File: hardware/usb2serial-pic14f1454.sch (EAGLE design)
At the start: 14 parts, among them IC1 PIC16F1454, IC2 LP2950-33, J1 USB-SHIELD-A-H, J2 J2

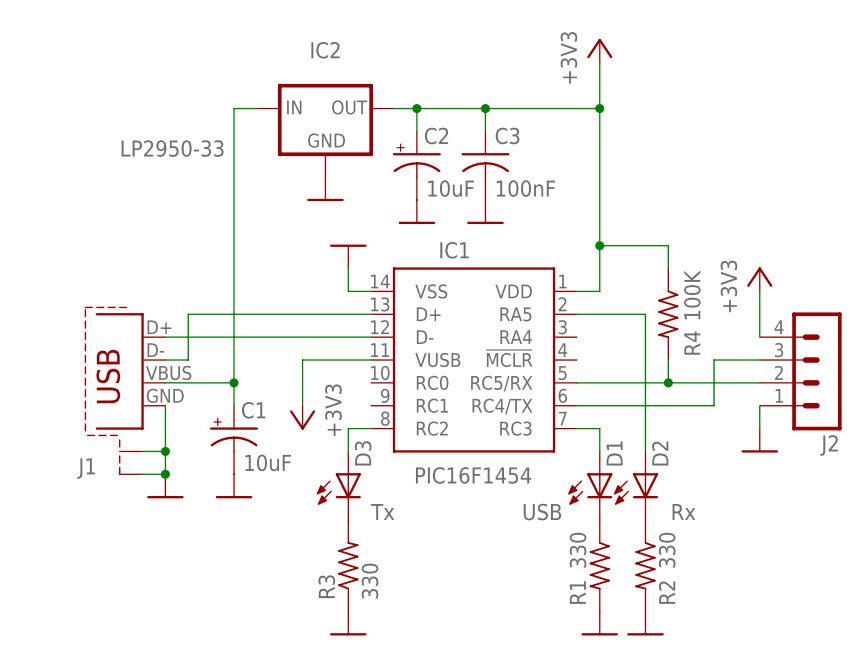
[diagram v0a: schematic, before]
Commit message: Cleanup
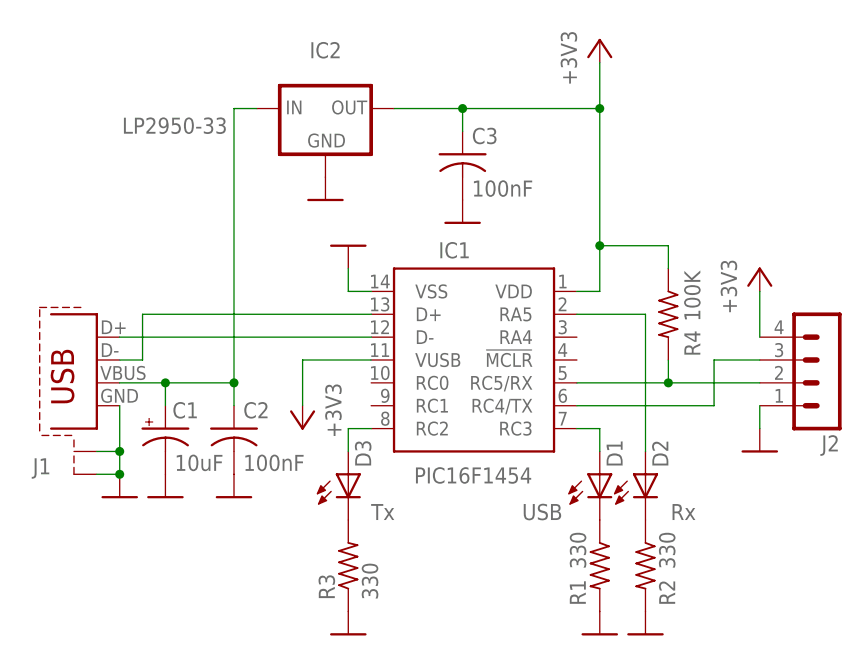
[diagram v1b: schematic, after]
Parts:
- C2: value 10uF -> 100nF; device rcl:CPOL-USE2-4 -> rcl:C-US050-025X075
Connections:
- net +3V3: no longer C2.+
- net GND: now also C2.2; no longer C2.-
- net N$6: now also C2.1
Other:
- moved on the sheet: C1, C3, J1
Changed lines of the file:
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@@
 <part name="D1" library="led" deviceset="LED" device="5MM"/>
 <part name="GND6" library="SparkFun" deviceset="GND" device=""/>
-<part name="GND7" library="supply1" deviceset="GND" device=""/>
-<part name="C2" library="rcl" deviceset="CPOL-US" device="E2-4" value="10uF"/>
 <part name="C3" library="rcl" deviceset="C-US" device="050-025X075" value="100nF"/>
 <part name="C1" library="rcl" deviceset="CPOL-US" device="E2-4" value="10uF"/>
@@
 <part name="R4" library="rcl" deviceset="R-US_" device="0207/10" value="100K"/>
 <part name="GND9" library="supply1" deviceset="GND" device=""/>
+<part name="C2" library="rcl" deviceset="C-US" device="050-025X075" value="100nF"/>
+<part name="GND10" library="supply1" deviceset="GND" device=""/>
 </parts>
 <sheets>
@@
 </plain>
 <instances>
-<instance part="GND15" gate="1" x="20.32" y="25.4" smashed="yes"/>
-<instance part="J1" gate="G$1" x="17.78" y="38.1" smashed="yes" rot="MR0">
-<attribute name="NAME" x="12.7" y="27.94" size="1.778" layer="95" rot="MR0"/>
-</instance>
-<instance part="GND1" gate="1" x="27.94" y="25.4" smashed="yes"/>
+<instance part="GND15" gate="1" x="15.24" y="25.4" smashed="yes"/>
+<instance part="J1" gate="G$1" x="12.7" y="38.1" smashed="yes" rot="MR0">
+<attribute name="NAME" x="7.62" y="27.94" size="1.778" layer="95" rot="MR0"/>
+</instance>
+<instance part="GND1" gate="1" x="20.32" y="25.4" smashed="yes"/>
 <instance part="J2" gate="1" x="93.98" y="40.64" smashed="yes" rot="MR0">
 <attribute name="VALUE" x="95.25" y="30.48" size="1.778" layer="96" rot="MR0"/>
@@
 </instance>
 <instance part="GND6" gate="1" x="38.1" y="58.42" smashed="yes"/>
-<instance part="GND7" gate="1" x="48.26" y="55.88" smashed="yes"/>
-<instance part="C2" gate="G$1" x="48.26" y="63.5" smashed="yes">
-<attribute name="NAME" x="49.022" y="64.643" size="1.778" layer="95"/>
-<attribute name="VALUE" x="49.276" y="58.801" size="1.778" layer="96"/>
-</instance>
-<instance part="C3" gate="G$1" x="55.88" y="63.5" smashed="yes">
-<attribute name="NAME" x="56.896" y="64.643" size="1.778" layer="95"/>
-<attribute name="VALUE" x="56.896" y="58.801" size="1.778" layer="96"/>
-</instance>
-<instance part="C1" gate="G$1" x="27.94" y="33.02" smashed="yes">
-<attribute name="NAME" x="28.702" y="34.163" size="1.778" layer="95"/>
-<attribute name="VALUE" x="28.956" y="28.321" size="1.778" layer="96"/>
+<instance part="C3" gate="G$1" x="53.34" y="63.5" smashed="yes">
+<attribute name="NAME" x="54.356" y="64.643" size="1.778" layer="95"/>
+<attribute name="VALUE" x="54.356" y="58.801" size="1.778" layer="96"/>
+</instance>
+<instance part="C1" gate="G$1" x="20.32" y="33.02" smashed="yes">
+<attribute name="NAME" x="21.082" y="34.163" size="1.778" layer="95"/>
+<attribute name="VALUE" x="21.336" y="28.321" size="1.778" layer="96"/>
 </instance>
 <instance part="+3V4" gate="G$1" x="35.56" y="33.02" rot="R180"/>
@@
 <instance part="IC2" gate="1" x="38.1" y="68.58" smashed="yes">
 <attribute name="NAME" x="36.322" y="74.168" size="1.778" layer="95"/>
-<attribute name="VALUE" x="15.24" y="63.246" size="1.778" layer="96"/>
+<attribute name="VALUE" x="15.494" y="65.786" size="1.778" layer="96"/>
 </instance>
 <instance part="GND4" gate="1" x="40.64" y="10.16" smashed="yes"/>
@@
 <attribute name="VALUE" x="77.978" y="50.546" size="1.778" layer="96" rot="R270"/>
 </instance>
-<instance part="GND9" gate="1" x="55.88" y="55.88" smashed="yes"/>
+<instance part="GND9" gate="1" x="53.34" y="55.88" smashed="yes"/>
+<instance part="C2" gate="G$1" x="27.94" y="33.02" smashed="yes">
+<attribute name="NAME" x="28.956" y="34.163" size="1.778" layer="95"/>
+<attribute name="VALUE" x="28.956" y="28.321" size="1.778" layer="96"/>
+</instance>
+<instance part="GND10" gate="1" x="27.94" y="25.4" smashed="yes"/>
 </instances>
 <busses>
@@
 <segment>
 <pinref part="J1" gate="G$1" pin="GND"/>
-<wire x1="20.32" y1="35.56" x2="20.32" y2="30.48" width="0.1524" layer="91"/>
+<wire x1="15.24" y1="35.56" x2="15.24" y2="30.48" width="0.1524" layer="91"/>
 <pinref part="GND15" gate="1" pin="GND"/>
 <pinref part="J1" gate="G$1" pin="S1"/>
-<wire x1="20.32" y1="30.48" x2="20.32" y2="27.94" width="0.1524" layer="91"/>
-<wire x1="17.78" y1="30.48" x2="20.32" y2="30.48" width="0.1524" layer="91"/>
-<junction x="20.32" y="30.48"/>
+<wire x1="15.24" y1="30.48" x2="15.24" y2="27.94" width="0.1524" layer="91"/>
+<wire x1="12.7" y1="30.48" x2="15.24" y2="30.48" width="0.1524" layer="91"/>
+<junction x="15.24" y="30.48"/>
 <pinref part="J1" gate="G$1" pin="S2"/>
-<wire x1="17.78" y1="27.94" x2="20.32" y2="27.94" width="0.1524" layer="91"/>
-<junction x="20.32" y="27.94"/>
+<wire x1="12.7" y1="27.94" x2="15.24" y2="27.94" width="0.1524" layer="91"/>
+<junction x="15.24" y="27.94"/>
 </segment>
 <segment>
@@
 </segment>
 <segment>
-<pinref part="C2" gate="G$1" pin="-"/>
-<pinref part="GND7" gate="1" pin="GND"/>
-</segment>
-<segment>
 <pinref part="C3" gate="G$1" pin="2"/>
 <pinref part="GND9" gate="1" pin="GND"/>
@@
 <pinref part="IC2" gate="1" pin="GND"/>
 </segment>
+<segment>
+<pinref part="C2" gate="G$1" pin="2"/>
+<pinref part="GND10" gate="1" pin="GND"/>
+</segment>
 </net>
 <net name="N$1" class="0">
 <segment>
 <pinref part="J1" gate="G$1" pin="D-"/>
-<wire x1="20.32" y1="40.64" x2="22.86" y2="40.64" width="0.1524" layer="91"/>
-<wire x1="22.86" y1="40.64" x2="22.86" y2="45.72" width="0.1524" layer="91"/>
+<wire x1="15.24" y1="40.64" x2="17.78" y2="40.64" width="0.1524" layer="91"/>
+<wire x1="17.78" y1="40.64" x2="17.78" y2="45.72" width="0.1524" layer="91"/>
 <pinref part="IC1" gate="G$1" pin="D+"/>
-<wire x1="22.86" y1="45.72" x2="43.18" y2="45.72" width="0.1524" layer="91"/>
+<wire x1="17.78" y1="45.72" x2="43.18" y2="45.72" width="0.1524" layer="91"/>
 </segment>
 </net>
 <net name="N$2" class="0">
 <segment>
-<wire x1="43.18" y1="43.18" x2="20.32" y2="43.18" width="0.1524" layer="91"/>
+<wire x1="43.18" y1="43.18" x2="15.24" y2="43.18" width="0.1524" layer="91"/>
 <pinref part="J1" gate="G$1" pin="D+"/>
 <pinref part="IC1" gate="G$1" pin="D-"/>
@@
 <net name="+3V3" class="0">
 <segment>
-<pinref part="C2" gate="G$1" pin="+"/>
 <pinref part="C3" gate="G$1" pin="1"/>
 <pinref part="IC1" gate="G$1" pin="VDD"/>
-<wire x1="68.58" y1="68.58" x2="55.88" y2="68.58" width="0.1524" layer="91"/>
-<wire x1="55.88" y1="68.58" x2="48.26" y2="68.58" width="0.1524" layer="91"/>
-<wire x1="48.26" y1="68.58" x2="45.72" y2="68.58" width="0.1524" layer="91"/>
+<wire x1="68.58" y1="68.58" x2="53.34" y2="68.58" width="0.1524" layer="91"/>
+<wire x1="53.34" y1="68.58" x2="45.72" y2="68.58" width="0.1524" layer="91"/>
 <wire x1="66.04" y1="48.26" x2="68.58" y2="48.26" width="0.1524" layer="91"/>
 <wire x1="68.58" y1="48.26" x2="68.58" y2="53.34" width="0.1524" layer="91"/>
@@
 <pinref part="R4" gate="G$1" pin="1"/>
 <wire x1="76.2" y1="53.34" x2="76.2" y2="50.8" width="0.1524" layer="91"/>
-<wire x1="48.26" y1="66.04" x2="48.26" y2="68.58" width="0.1524" layer="91"/>
-<junction x="48.26" y="68.58"/>
-<wire x1="55.88" y1="66.04" x2="55.88" y2="68.58" width="0.1524" layer="91"/>
-<junction x="55.88" y="68.58"/>
+<wire x1="53.34" y1="66.04" x2="53.34" y2="68.58" width="0.1524" layer="91"/>
+<junction x="53.34" y="68.58"/>
 </segment>
 <segment>
@@
 <segment>
 <pinref part="J1" gate="G$1" pin="VBUS"/>
-<wire x1="20.32" y1="38.1" x2="27.94" y2="38.1" width="0.1524" layer="91"/>
-<wire x1="27.94" y1="38.1" x2="27.94" y2="35.56" width="0.1524" layer="91"/>
-<junction x="27.94" y="38.1"/>
-<wire x1="27.94" y1="38.1" x2="27.94" y2="68.58" width="0.1524" layer="91"/>
-<wire x1="27.94" y1="68.58" x2="30.48" y2="68.58" width="0.1524" layer="91"/>
+<wire x1="15.24" y1="38.1" x2="20.32" y2="38.1" width="0.1524" layer="91"/>
+<wire x1="20.32" y1="38.1" x2="20.32" y2="35.56" width="0.1524" layer="91"/>
+<junction x="20.32" y="38.1"/>
 <pinref part="C1" gate="G$1" pin="+"/>
 <pinref part="IC2" gate="1" pin="IN"/>
-</segment>
-</net>
+<wire x1="20.32" y1="38.1" x2="27.94" y2="38.1" width="0.1524" layer="91"/>
+<pinref part="C2" gate="G$1" pin="1"/>
+<wire x1="27.94" y1="38.1" x2="27.94" y2="35.56" width="0.1524" layer="91"/>
+<wire x1="27.94" y1="38.1" x2="27.94" y2="68.58" width="0.1524" layer="91"/>
+<junction x="27.94" y="38.1"/>
+<wire x1="27.94" y1="68.58" x2="30.48" y2="68.58" width="0.1524" layer="91"/>
+</segment>
+</net>
